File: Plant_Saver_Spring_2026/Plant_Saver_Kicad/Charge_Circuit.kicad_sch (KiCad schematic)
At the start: 23 parts, among them J1 1.25mm, Q1 ISP12DP06NMXTSA1, Q2 G09P02L, Q3 G09P02L, Q4 G09P02L, Q5 G09P02L, Q6 G09P02L, Q7 G09P02L, Q8 G09P02L, SW7 SA72SB0, U10 DW03C, U11 CDBA140SL-HF, U12 CDBA140SL-HF

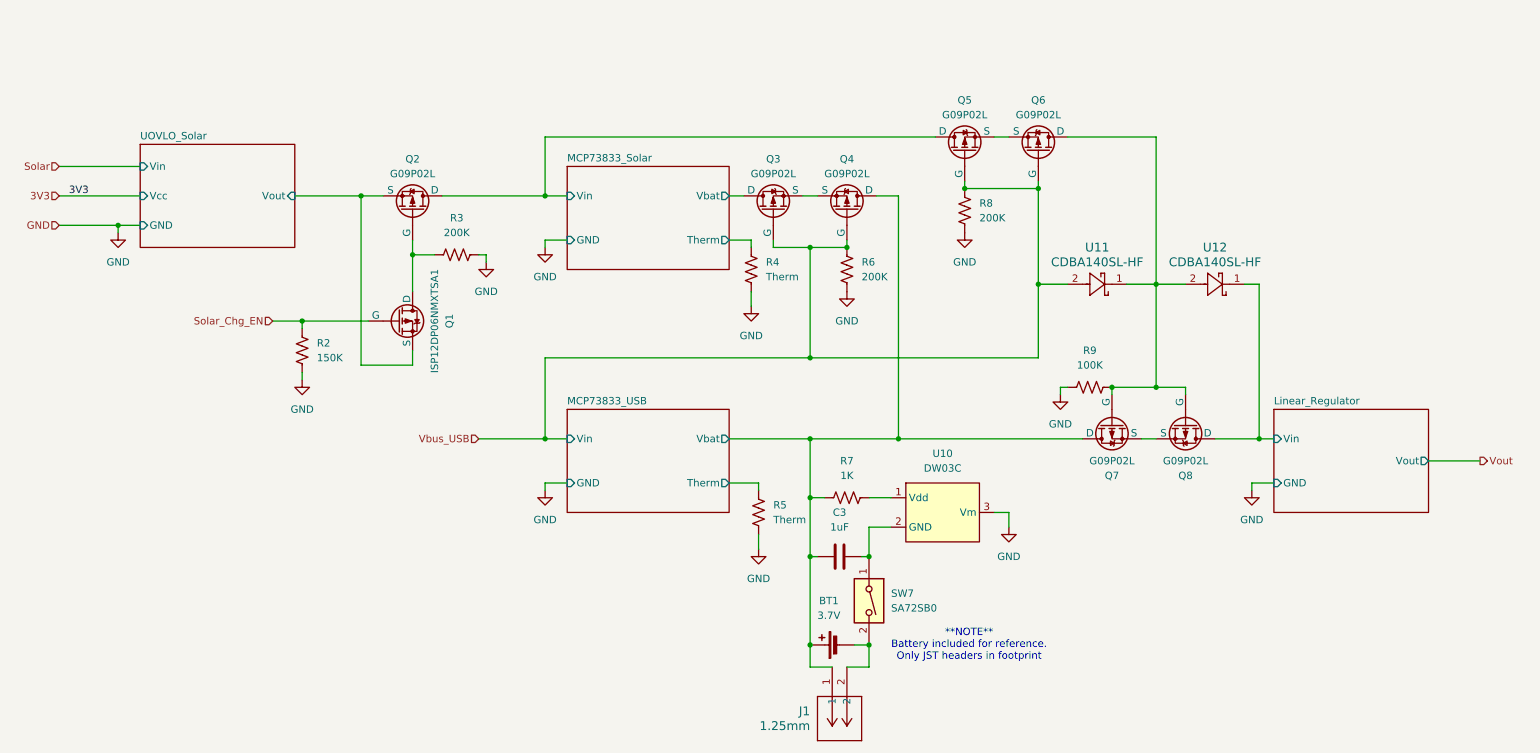
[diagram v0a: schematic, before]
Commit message: Found NTC Thermistor
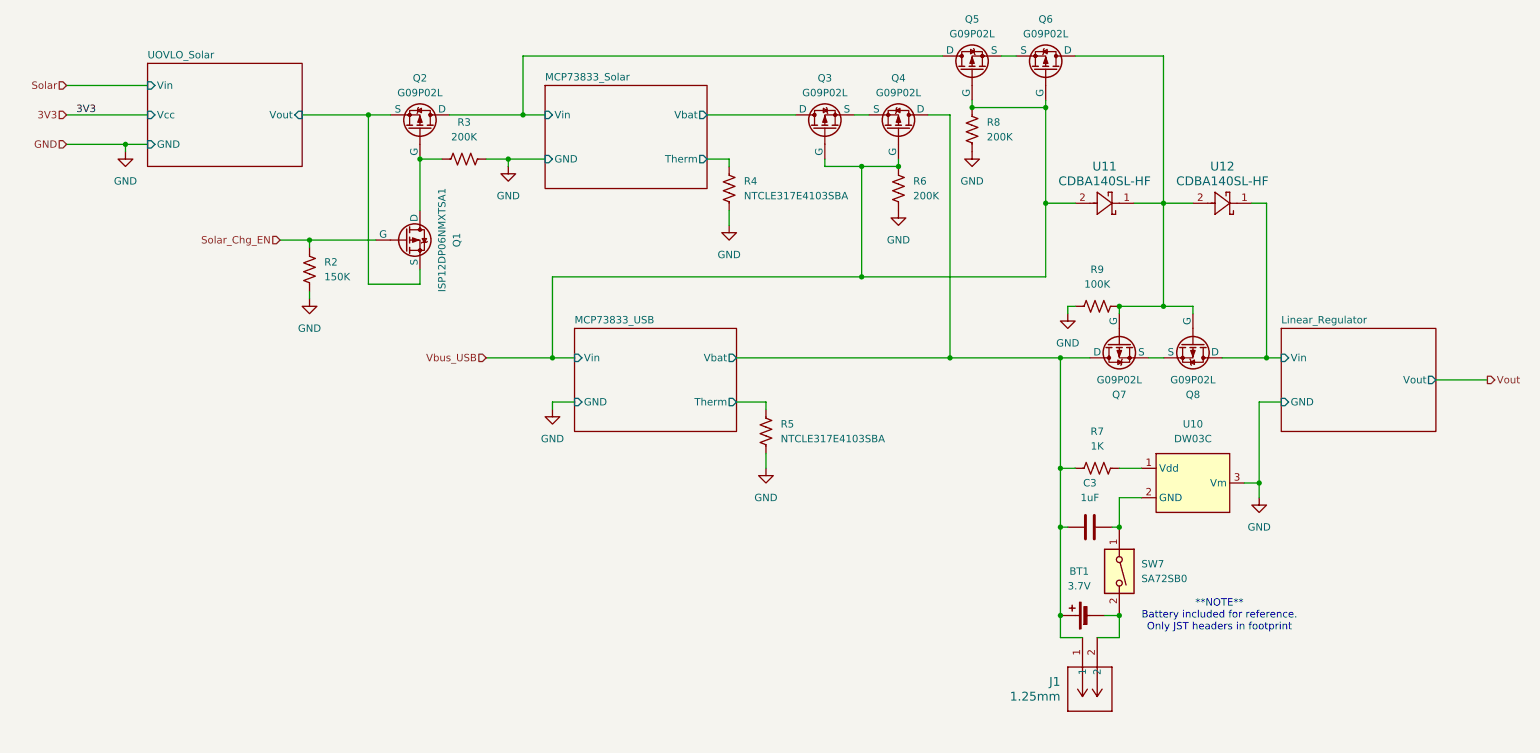
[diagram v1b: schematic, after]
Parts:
- R4, R5: value Therm -> NTCLE317E4103SBA
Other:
- moved on the sheet: BT1, C3, J1, Q1, Q2, Q3, Q4, Q5, Q6, Q7, Q8, R2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
